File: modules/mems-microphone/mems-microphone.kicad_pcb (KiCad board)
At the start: 2 copper layers, 10 x 12.7 mm, 6 parts

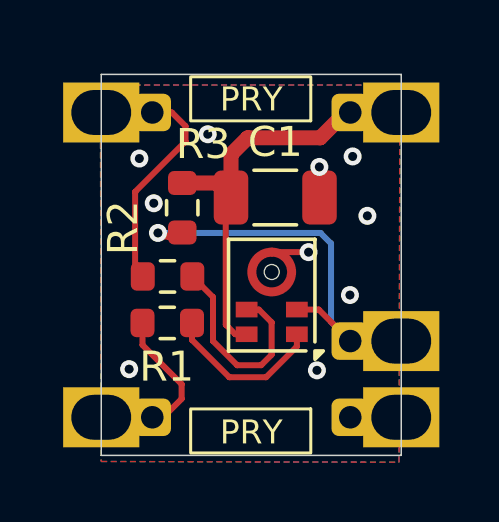
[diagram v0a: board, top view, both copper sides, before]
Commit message: Updating all modules
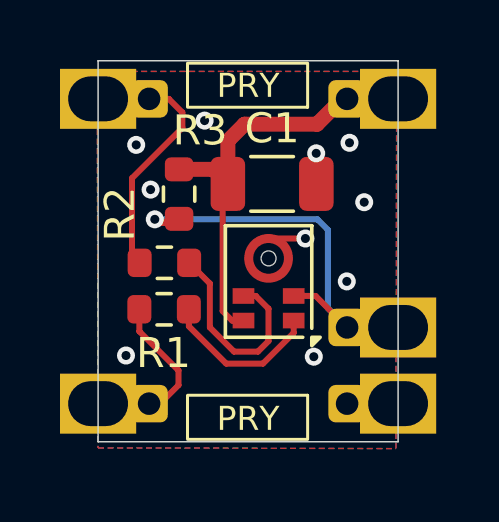
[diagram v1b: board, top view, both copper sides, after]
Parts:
- moved M1 0.47 mm to (61.8, 47.2)
- moved C1 0.47 mm to (62.6, 44.9)
- moved MK1 0.47 mm to (62.5, 48.2)
- moved R1 0.47 mm to (59.0, 49.1)
- moved R2 0.47 mm to (59.1, 47.6)
- moved R3 0.47 mm to (59.5, 45.3)
